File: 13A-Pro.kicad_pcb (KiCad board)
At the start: 2 copper layers, 81 x 81 mm, 30 parts, among them SW1 SW_Push, U1 ProMicro

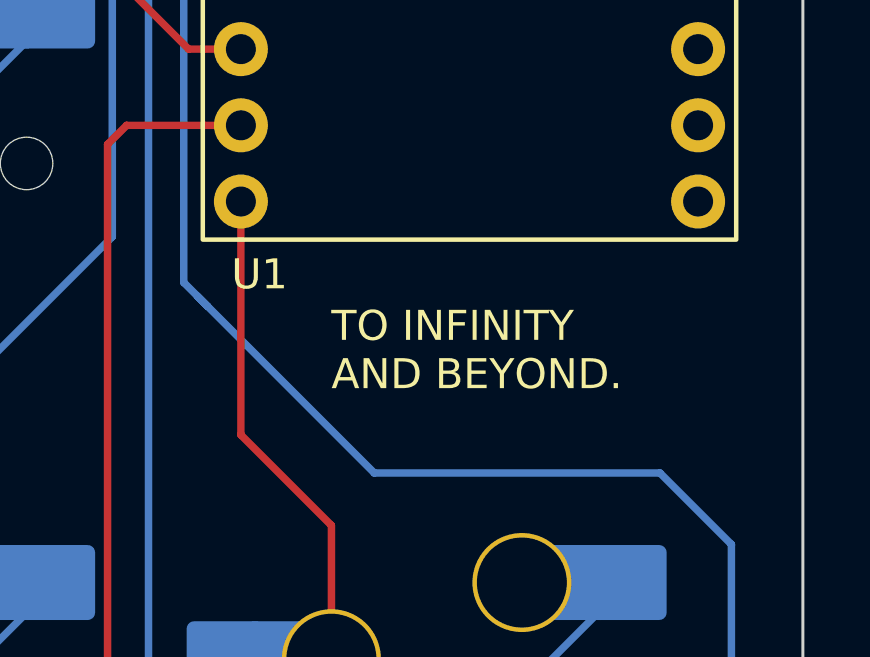
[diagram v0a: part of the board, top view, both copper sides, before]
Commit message: Case, PCB, Firmware update
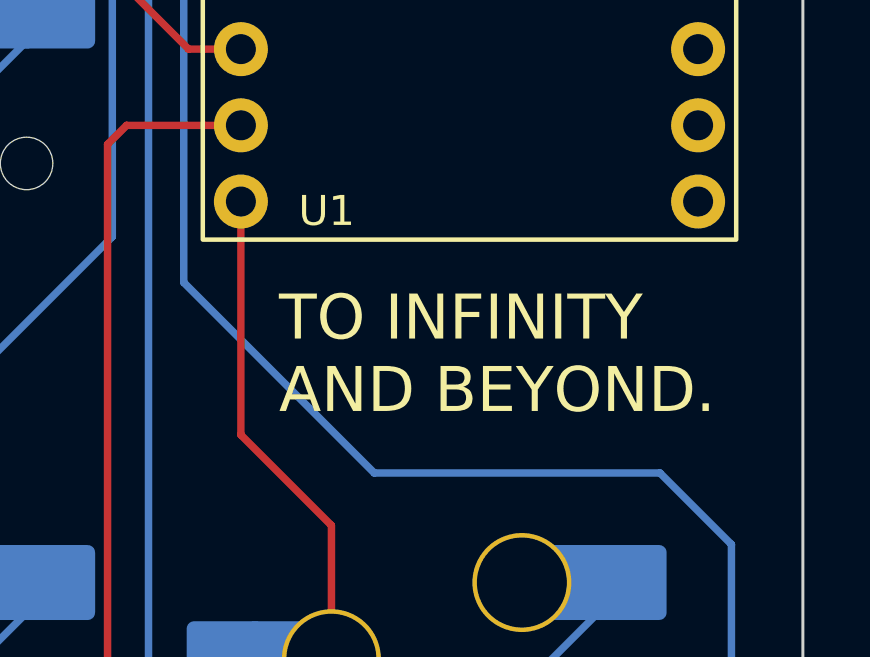
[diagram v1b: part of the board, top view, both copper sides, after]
